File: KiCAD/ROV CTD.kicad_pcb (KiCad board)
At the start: 2 copper layers, 99.1 x 23.4 mm, 37 parts, among them J1 Conn_Coaxial, J10 1Wire1, J11 1Wire2, J12 1Wire3, J13 Interface, J14 Interface, J15 Conn_01x07_Pin, J6 Main In, M1 EZO-EC, U2 ATtiny1614-Arduino, U3 AP63205WU, U6 MAX3072E

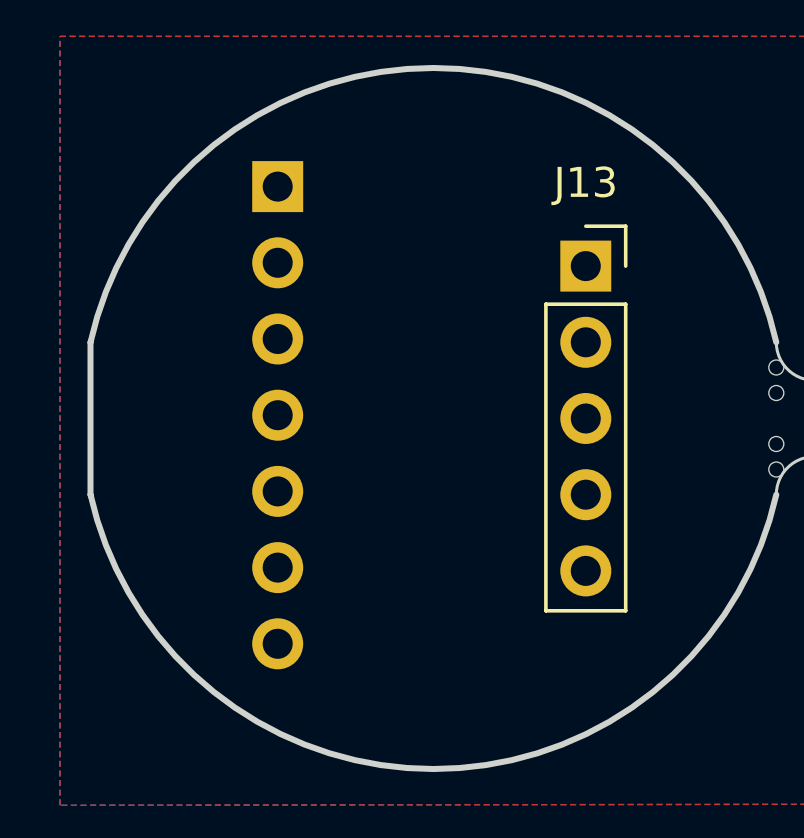
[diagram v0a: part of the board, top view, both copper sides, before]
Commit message: .
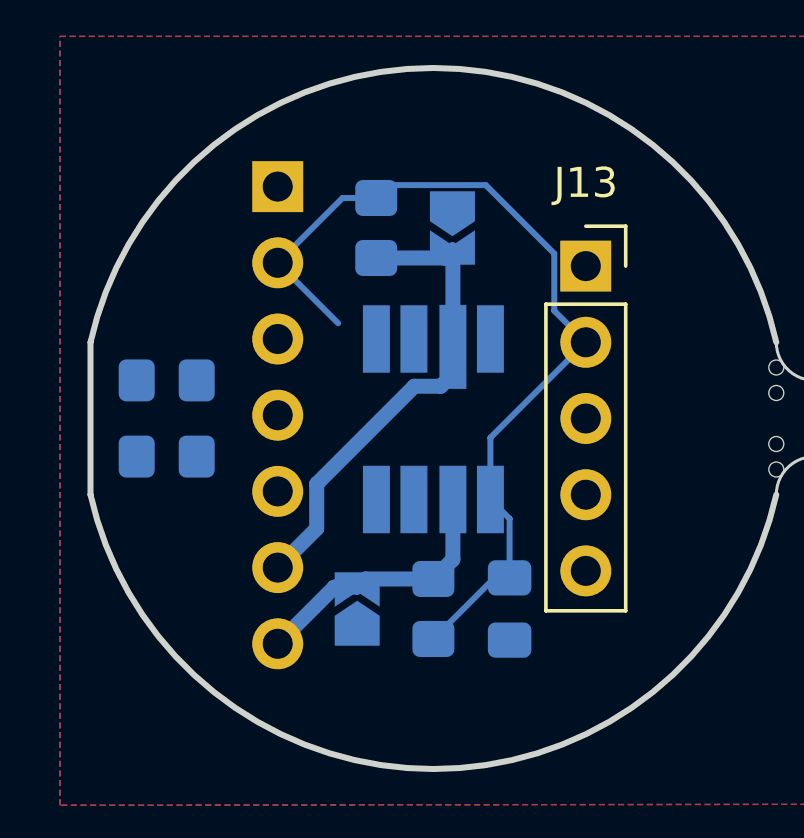
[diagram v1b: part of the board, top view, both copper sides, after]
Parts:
- added C7: 100nF, Capacitor_SMD:C_0805_2012Metric_Pad1.18x1.45mm_HandSolder, B.Cu at (142.2, 82.5)
- added JP3: RX, Jumper:SolderJumper-2_P1.3mm_Open_TrianglePad1.0x1.5mm, B.Cu at (137.2, 82.5)
- added JP4: RX, Jumper:SolderJumper-2_P1.3mm_Open_TrianglePad1.0x1.5mm, B.Cu at (140.3, 69.8)
- added M2: MS5803-14BA, KiCad Footprints:MS5803-14BA, B.Cu at (139.7, 76.2)
- added R12: 10k, Resistor_SMD:R_0805_2012Metric_Pad1.20x1.40mm_HandSolder, B.Cu at (139.7, 82.5)
- added R13: 10k, Resistor_SMD:R_0805_2012Metric_Pad1.20x1.40mm_HandSolder, B.Cu at (137.8, 69.8)
- added R14: 2k2, Resistor_SMD:R_0805_2012Metric_Pad1.20x1.40mm_HandSolder, B.Cu at (130.8, 74.9)
- added R15: 2k2, Resistor_SMD:R_0805_2012Metric_Pad1.20x1.40mm_HandSolder, B.Cu at (130.8, 77.5)
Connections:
- J13 pad 1: unconnected-(J13-Pin_1-Pad1) -> GND
- J13 pad 2: unconnected-(J13-Pin_2-Pad2) -> +3V3
- J14 pad 1: unconnected-(J14-Pin_1-Pad1) -> GND
- J14 pad 2: unconnected-(J14-Pin_2-Pad2) -> +3V3
- J15 pad 1: unconnected-(J15-Pin_1-Pad1) -> GND
- J15 pad 2: unconnected-(J15-Pin_2-Pad2) -> +3V3
- J15 pad 3: unconnected-(J15-Pin_3-Pad3) -> /SDA/SDI
- J15 pad 4: unconnected-(J15-Pin_4-Pad4) -> /SCL/SCLK
- J15 pad 5: unconnected-(J15-Pin_5-Pad5) -> /SDO
- J15 pad 6: unconnected-(J15-Pin_6-Pad6) -> /AD/CS
- J15 pad 7: unconnected-(J15-Pin_7-Pad7) -> /PS
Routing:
- net +3V3: track 0.00 -> 31.2 mm
- net /AD/CS: track 0.00 -> 16.2 mm
- net /PS: track 0.00 -> 9.00 mm

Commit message: .
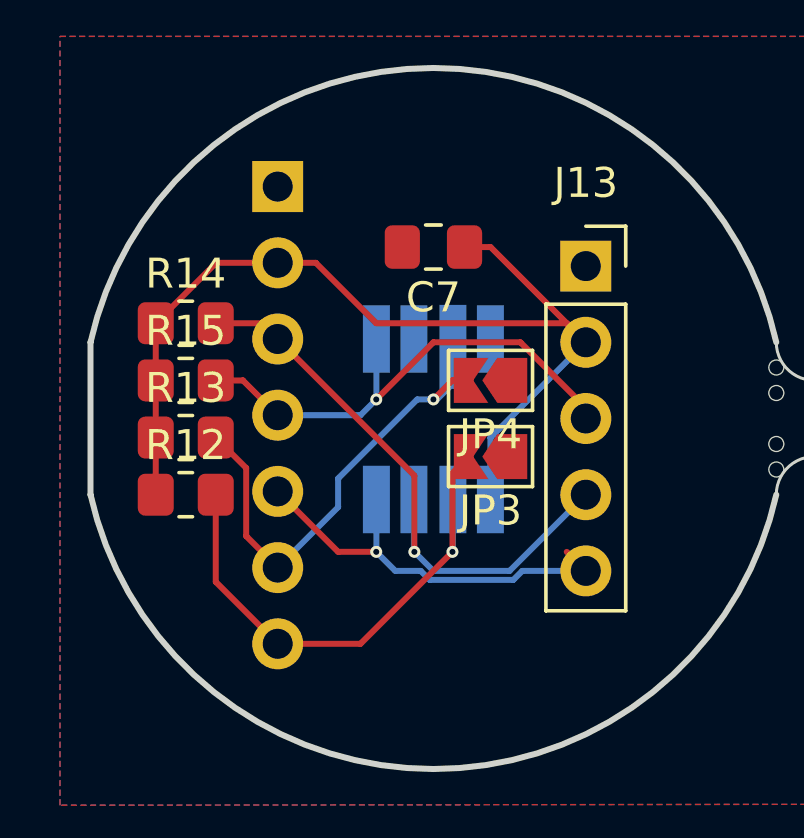
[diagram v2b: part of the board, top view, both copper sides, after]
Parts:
- C7, JP3, JP4, R12, R13, R14, R15: moved to F.Cu
- moved C7 12.3 mm to (139.7, 70.5), turned to 180 degrees
- moved R13 9.44 mm to (131.4, 76.8), turned to 0 degrees
- moved R12 9.09 mm to (131.4, 78.7), turned to 0 degrees
- moved JP3 6.75 mm to (141.6, 77.5), turned to 180 degrees
- moved JP4 5.24 mm to (141.6, 74.9), turned to 180 degrees
- moved R15 2.62 mm to (131.4, 74.9)
- moved R14 2.01 mm to (131.4, 73.0)
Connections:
- J13 pad 3: unconnected-(J13-Pin_3-Pad3) -> /SCL/SCLK
- J13 pad 4: unconnected-(J13-Pin_4-Pad4) -> /SDA/SDI
- J13 pad 5: unconnected-(J13-Pin_5-Pad5) -> /SDO
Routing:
- net /SDA/SDI: track 0.00 -> 20.0 mm, vias 0 -> 1
- net /SCL/SCLK: track 0.00 -> 17.1 mm, vias 0 -> 1
- net /SDO: track 0.00 -> 14.6 mm, vias 0 -> 1
- net /PS: track 9.00 -> 18.1 mm, vias 0 -> 1
- net +3V3: track 31.2 -> 34.9 mm
- net /AD/CS: track 16.2 -> 16.8 mm, vias 0 -> 1
